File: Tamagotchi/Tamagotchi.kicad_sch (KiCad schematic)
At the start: 15 parts, among them SW1 SW_Push, SW2 SW_Push, SW3 SW_Push, U1 XIAO-ESP32-C6-DIP, U2 DM-OLED096-636

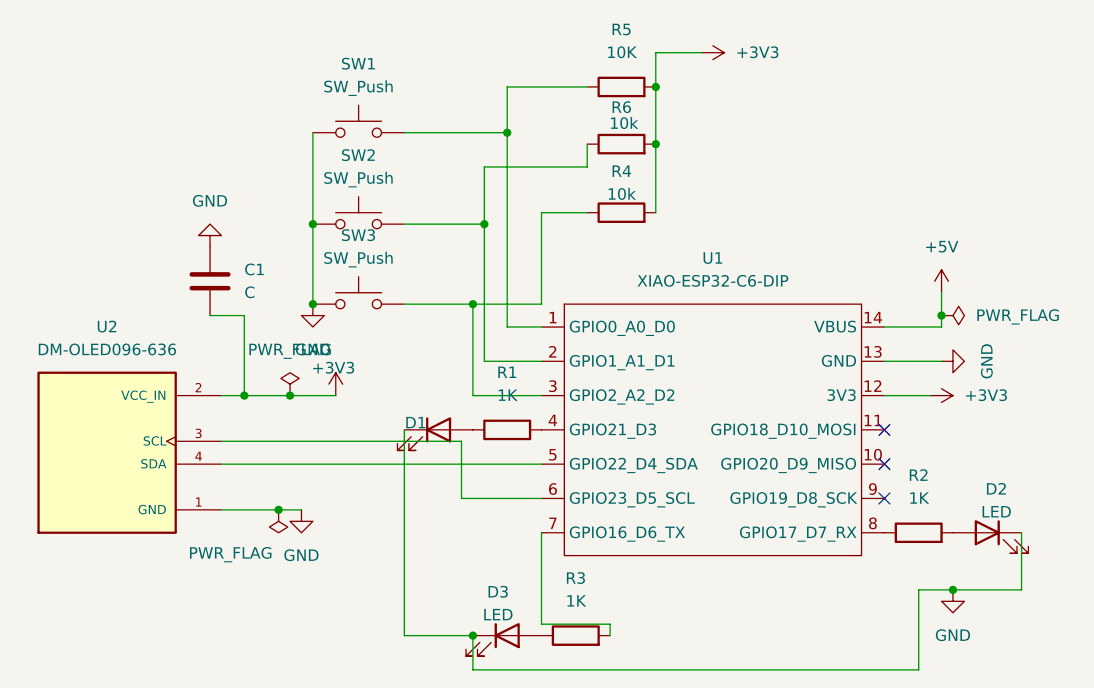
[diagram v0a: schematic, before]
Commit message: testing out if my github deskstop still functions
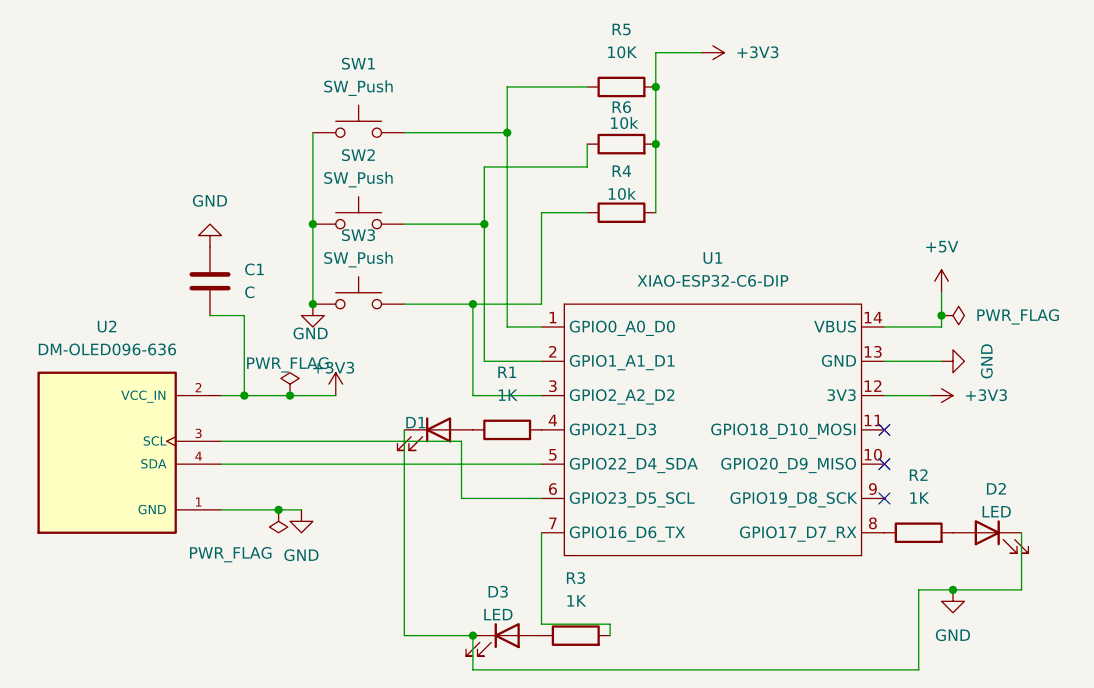
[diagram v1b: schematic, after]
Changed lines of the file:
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@@
 		(in_pos_files yes)
 		(dnp no)
-		(fields_autoplaced yes)
 		(property "Reference" "#FLG01"
 			(at 101.6 85.725 0)
@@
 		)
 		(property "Value" "PWR_FLAG"
-			(at 101.6 82.55 0)
+			(at 101.346 84.074 0)
 			(show_name no)
 			(do_not_autoplace no)
@@
 				(path "/dd5d29a8-0ca1-4c75-a105-470d6b907a46"
 					(reference "#FLG01")
-					(unit 1)
-				)
-			)
-		)
-	)
-	(symbol
-		(lib_id "DM-OLED096-636:DM-OLED096-636")
-		(at 81.28 95.25 0)
-		(unit 1)
-		(body_style 1)
-		(exclude_from_sim no)
-		(in_bom yes)
-		(on_board yes)
-		(in_pos_files yes)
-		(dnp no)
-		(property "Reference" "U2"
-			(at 81.28 80.01 0)
-			(show_name no)
-			(do_not_autoplace no)
-			(effects
-				(font
-					(size 1.27 1.27)
-				)
-			)
-		)
-		(property "Value" "DM-OLED096-636"
-			(at 81.28 82.55 0)
-			(show_name no)
-			(do_not_autoplace no)
-			(effects
-				(font
-					(size 1.27 1.27)
-				)
-			)
-		)
-		(property "Footprint" "DM-OLED096-636 (1):MODULE_DM-OLED096-636"
-			(at 81.28 95.25 0)
-			(hide yes)
-			(show_name no)
-			(do_not_autoplace no)
-			(effects
-				(font
-					(size 1.27 1.27)
-				)
-				(justify bottom)
-			)
-		)
-		(property "Datasheet" ""
-			(at 81.28 95.25 0)
-			(hide yes)
-			(show_name no)
-			(do_not_autoplace no)
-			(effects
-				(font
-					(size 1.27 1.27)
-				)
-			)
-		)
-		(property "Description" "0.96” 128 X 64 MONOCHROME GRAPHIC OLED DISPLAY MODULE - I2C"
-			(at 81.28 95.25 0)
-			(hide yes)
-			(show_name no)
-			(do_not_autoplace no)
-			(effects
-				(font
-					(size 1.27 1.27)
-				)
-				(justify bottom)
-			)
-		)
-		(property "MF" "Display Module"
-			(at 81.28 95.25 0)
-			(hide yes)
-			(show_name no)
-			(do_not_autoplace no)
-			(effects
-				(font
-					(size 1.27 1.27)
-				)
-				(justify bottom)
-			)
-		)
-		(property "MAXIMUM_PACKAGE_HEIGHT" "11.3 mm"
-			(at 81.28 95.25 0)
-			(hide yes)
-			(show_name no)
-			(do_not_autoplace no)
-			(effects
-				(font
-					(size 1.27 1.27)
-				)
-				(justify bottom)
-			)
-		)
-		(property "Package" "Package"
-			(at 81.28 95.25 0)
-			(hide yes)
-			(show_name no)
-			(do_not_autoplace no)
-			(effects
-				(font
-					(size 1.27 1.27)
-				)
-				(justify bottom)
-			)
-		)
-		(property "Price" "None"
-			(at 81.28 95.25 0)
-			(hide yes)
-			(show_name no)
-			(do_not_autoplace no)
-			(effects
-				(font
-					(size 1.27 1.27)
-				)
-				(justify bottom)
-			)
-		)
-		(property "Check_prices" "https://www.snapeda.com/parts/DM-OLED096-636/Display+Module/view-part/?ref=eda"
-			(at 81.28 95.25 0)
-			(hide yes)
-			(show_name no)
-			(do_not_autoplace no)
-			(effects
-				(font
-					(size 1.27 1.27)
-				)
-				(justify bottom)
-			)
-		)
-		(property "STANDARD" "Manufacturer Recommendations"
-			(at 81.28 95.25 0)
-			(hide yes)
-			(show_name no)
-			(do_not_autoplace no)
-			(effects
-				(font
-					(size 1.27 1.27)
-				)
-				(justify bottom)
-			)
-		)
-		(property "PARTREV" "2018-09-10"
-			(at 81.28 95.25 0)
-			(hide yes)
-			(show_name no)
-			(do_not_autoplace no)
-			(effects
-				(font
-					(size 1.27 1.27)
-				)
-				(justify bottom)
-			)
-		)
-		(property "SnapEDA_Link" "https://www.snapeda.com/parts/DM-OLED096-636/Display+Module/view-part/?ref=snap"
-			(at 81.28 95.25 0)
-			(hide yes)
-			(show_name no)
-			(do_not_autoplace no)
-			(effects
-				(font
-					(size 1.27 1.27)
-				)
-				(justify bottom)
-			)
-		)
-		(property "MP" "DM-OLED096-636"
-			(at 81.28 95.25 0)
-			(hide yes)
-			(show_name no)
-			(do_not_autoplace no)
-			(effects
-				(font
-					(size 1.27 1.27)
-				)
-				(justify bottom)
-			)
-		)
-		(property "Availability" "Not in stock"
-			(at 81.28 95.25 0)
-			(hide yes)
-			(show_name no)
-			(do_not_autoplace no)
-			(effects
-				(font
-					(size 1.27 1.27)
-				)
-				(justify bottom)
-			)
-		)
-		(property "MANUFACTURER" "Displaymodule"
-			(at 81.28 95.25 0)
-			(hide yes)
-			(show_name no)
-			(do_not_autoplace no)
-			(effects
-				(font
-					(size 1.27 1.27)
-				)
-				(justify bottom)
-			)
-		)
-		(pin "4"
-		)
-		(pin "3"
-		)
-		(pin "1"
-		)
-		(pin "2"
-		)
-		(instances
-			(project "Tamagotchi"
-				(path "/dd5d29a8-0ca1-4c75-a105-470d6b907a46"
-					(reference "U2")
 					(unit 1)
 				)
@@
 		)
 		(property "Value" "GND"
-			(at 104.14 82.55 0)
+			(at 103.886 80.772 0)
 			(show_name no)
 			(do_not_autoplace no)
@@
 					(unit 1)
 				)
+			)
+		)
+	)
+	(symbol
+		(lib_id "DM-OLED096-636:DM-OLED096-636")
+		(at 81.28 95.25 0)
+		(unit 1)
+		(body_style 1)
+		(exclude_from_sim no)
+		(in_bom yes)
+		(on_board yes)
+		(in_pos_files yes)
+		(dnp no)
+		(property "Reference" "U2"
+			(at 81.28 80.01 0)
+			(show_name no)
+			(do_not_autoplace no)
+			(effects
+				(font
+					(size 1.27 1.27)
+				)
+			)
+		)
+		(property "Value" "DM-OLED096-636"
+			(at 81.28 82.55 0)
+			(show_name no)
+			(do_not_autoplace no)
+			(effects
+				(font
+					(size 1.27 1.27)
+				)
+			)
+		)
+		(property "Footprint" "DM-OLED096-636 (1):MODULE_DM-OLED096-636"
+			(at 81.28 95.25 0)
+			(hide yes)
+			(show_name no)
+			(do_not_autoplace no)
+			(effects
+				(font
+					(size 1.27 1.27)
+				)
+				(justify bottom)
+			)
+		)
+		(property "Datasheet" ""
+			(at 81.28 95.25 0)
+			(hide yes)
+			(show_name no)
+			(do_not_autoplace no)
+			(effects
+				(font
+					(size 1.27 1.27)
+				)
+			)
+		)
+		(property "Description" "0.96” 128 X 64 MONOCHROME GRAPHIC OLED DISPLAY MODULE - I2C"
+			(at 81.28 95.25 0)
+			(hide yes)
+			(show_name no)
+			(do_not_autoplace no)
+			(effects
+				(font
+					(size 1.27 1.27)
+				)
+				(justify bottom)
+			)
+		)
+		(property "MF" "Display Module"
+			(at 81.28 95.25 0)
+			(hide yes)
+			(show_name no)
+			(do_not_autoplace no)
+			(effects
+				(font
+					(size 1.27 1.27)
+				)
+				(justify bottom)
+			)
+		)
+		(property "MAXIMUM_PACKAGE_HEIGHT" "11.3 mm"
+			(at 81.28 95.25 0)
+			(hide yes)
+			(show_name no)
+			(do_not_autoplace no)
+			(effects
+				(font
+					(size 1.27 1.27)
+				)
+				(justify bottom)
+			)
+		)
+		(property "Package" "Package"
+			(at 81.28 95.25 0)
+			(hide yes)
+			(show_name no)
+			(do_not_autoplace no)
+			(effects
+				(font
+					(size 1.27 1.27)
+				)
+				(justify bottom)
+			)
+		)
+		(property "Price" "None"
+			(at 81.28 95.25 0)
+			(hide yes)
+			(show_name no)
+			(do_not_autoplace no)
+			(effects
+				(font
+					(size 1.27 1.27)
+				)
+				(justify bottom)
+			)
+		)
+		(property "Check_prices" "https://www.snapeda.com/parts/DM-OLED096-636/Display+Module/view-part/?ref=eda"
+			(at 81.28 95.25 0)
+			(hide yes)
+			(show_name no)
+			(do_not_autoplace no)
+			(effects
+				(font
+					(size 1.27 1.27)
+				)
+				(justify bottom)
+			)
+		)
+		(property "STANDARD" "Manufacturer Recommendations"
+			(at 81.28 95.25 0)
+			(hide yes)
+			(show_name no)
+			(do_not_autoplace no)
+			(effects
+				(font
+					(size 1.27 1.27)
+				)
+				(justify bottom)
+			)
+		)
+		(property "PARTREV" "2018-09-10"
+			(at 81.28 95.25 0)
+			(hide yes)
+			(show_name no)
+			(do_not_autoplace no)
+			(effects
+				(font
+					(size 1.27 1.27)
+				)
+				(justify bottom)
+			)
+		)
+		(property "SnapEDA_Link" "https://www.snapeda.com/parts/DM-OLED096-636/Display+Module/view-part/?ref=snap"
+			(at 81.28 95.25 0)
+			(hide yes)
+			(show_name no)
+			(do_not_autoplace no)
+			(effects
+				(font
+					(size 1.27 1.27)
+				)
+				(justify bottom)
+			)
+		)
+		(property "MP" "DM-OLED096-636"
+			(at 81.28 95.25 0)
+			(hide yes)
+			(show_name no)
+			(do_not_autoplace no)
+			(effects
+				(font
+					(size 1.27 1.27)
+				)
+				(justify bottom)
+			)
+		)
+		(property "Availability" "Not in stock"
+			(at 81.28 95.25 0)
+			(hide yes)
+			(show_name no)
+			(do_not_autoplace no)
+			(effects
+				(font
+					(size 1.27 1.27)
+				)
+				(justify bottom)
+			)
+		)
+		(property "MANUFACTURER" "Displaymodule"
+			(at 81.28 95.25 0)
+			(hide yes)
+			(show_name no)
+			(do_not_autoplace no)
+			(effects
+				(font
+					(size 1.27 1.27)
+				)
+				(justify bottom)
+			)
+		)
+		(pin "4"
+		)
+		(pin "3"
+		)
+		(pin "1"
+		)
+		(pin "2"
+		)
+		(instances
+			(project "Tamagotchi"
+				(path "/dd5d29a8-0ca1-4c75-a105-470d6b907a46"
+					(reference "U2")
+					(unit 1)
+				)
